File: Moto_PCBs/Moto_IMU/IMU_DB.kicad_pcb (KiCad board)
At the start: 2 copper layers, 60 x 30 mm, 31 parts, among them J1 POWER IN, J2 CANBUS, J3 Conn_01x05_Pin 61300511121, U1 STM32F103C8Tx, U2 IAM-20680HP, U3 SN65HVD230

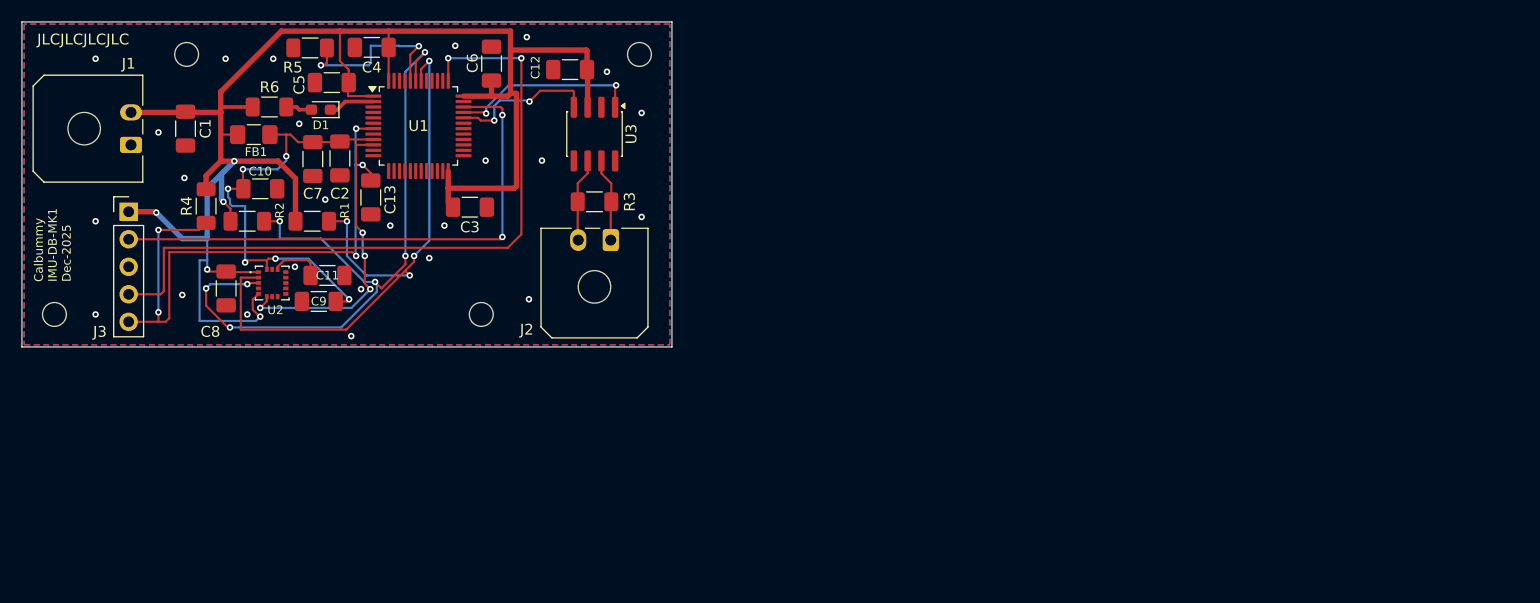
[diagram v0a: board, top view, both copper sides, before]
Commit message: Add files via upload
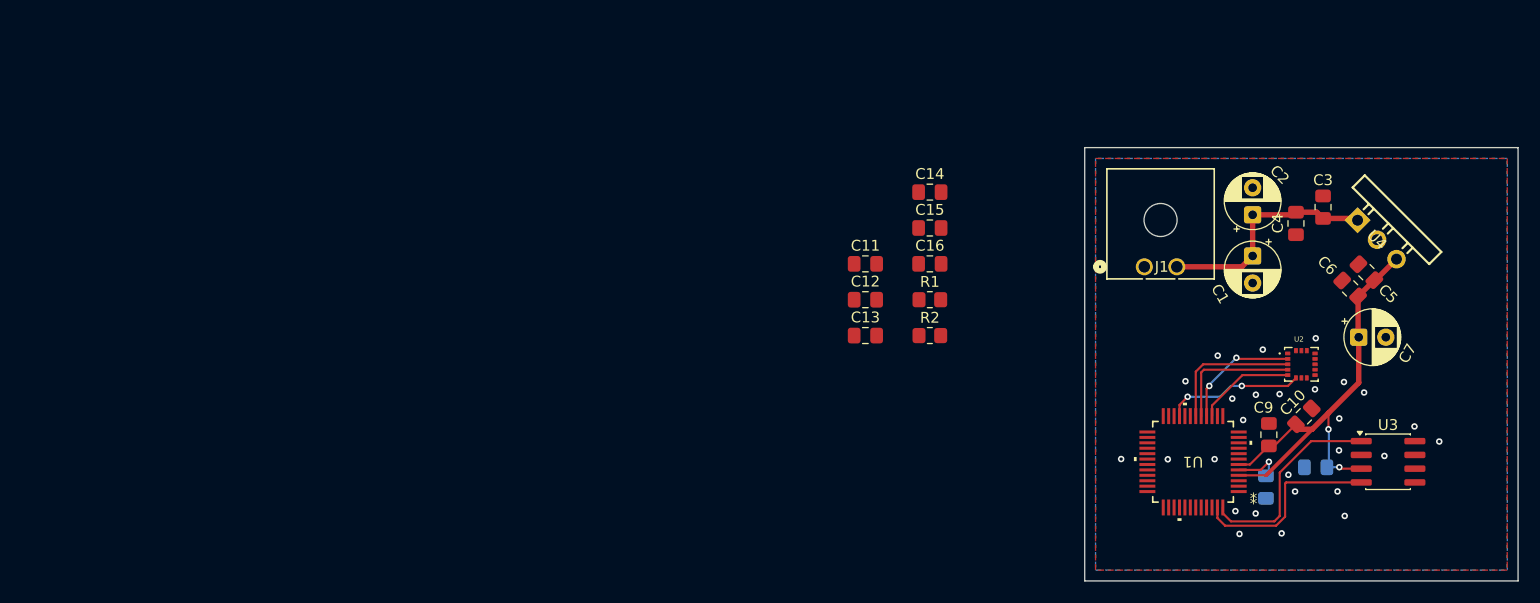
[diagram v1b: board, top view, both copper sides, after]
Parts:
- removed D1: SML-D12P8WT86C, LED_SMD:LED_0603_1608Metric_Pad1.05x0.95mm_HandSolder
- removed FB1: 742792113, Inductor_SMD:L_1206_3216Metric_Pad1.42x1.75mm_HandSolder
- removed J2: CANBUS, Connector_Molex:Molex_Micro-Fit_3.0_43650-0200_1x02_P3.00mm_Horizontal
- removed J3: Conn_01x05_Pin 61300511121, Connector_PinHeader_2.54mm:PinHeader_1x05_P2.54mm_Vertical
- removed R3: RC1206JR-07120RL - OPTIONAL TERM ONLY, Resistor_SMD:R_1206_3216Metric_Pad1.30x1.75mm_HandSolder
- removed R4, R5: RC1206FR-0710KL 10kOhm, Resistor_SMD:R_1206_3216Metric_Pad1.30x1.75mm_HandSolder
- removed R6: RNCP1206FTD1K00 1kOhm, Resistor_SMD:R_1206_3216Metric_Pad1.30x1.75mm_HandSolder
- removed REF** (x4): MountingHole_2.2mm_M2_DIN965, MountingHole:MountingHole_2.2mm_M2_DIN965
- added C14: 10nF, Capacitor_SMD:C_0805_2012Metric_Pad1.18x1.45mm_HandSolder, F.Cu at (108.2, 86.1)
- added C15: .1uF, Capacitor_SMD:C_0805_2012Metric_Pad1.18x1.45mm_HandSolder, F.Cu at (108.2, 89.4)
- added C16: 2.2uF, Capacitor_SMD:C_0805_2012Metric_Pad1.18x1.45mm_HandSolder, F.Cu at (108.2, 92.7)
- added C17: 100nF, Capacitor_SMD:C_0805_2012Metric_Pad1.18x1.45mm_HandSolder, B.Cu at (143.8, 111.5)
- added U4: TPSM84203EAB, TPSM84203EAB:EAB0003A, F.Cu at (149.5, 90.5)
- C1: value CL31B106KQHNFNE 10uF 6.3V -> 100uF; footprint Capacitor_SMD:C_1206_3216Metric_Pad1.33x1.80mm_HandSolder -> Capacitor_THT:CP_Radial_D5.0mm_P2.50mm
- C10: value 885012208013 1uF 10V -> 4.7uF; footprint Capacitor_SMD:C_1206_3216Metric_Pad1.33x1.80mm_HandSolder -> Capacitor_SMD:C_0805_2012Metric_Pad1.18x1.45mm_HandSolder
- C11: value 885012208009 .1uF 10V -> 4.7uF; footprint Capacitor_SMD:C_1206_3216Metric_Pad1.33x1.80mm_HandSolder -> Capacitor_SMD:C_0805_2012Metric_Pad1.18x1.45mm_HandSolder
- C12: value 885012208009 .1uF 10V -> 100nF; footprint Capacitor_SMD:C_1206_3216Metric_Pad1.33x1.80mm_HandSolder -> Capacitor_SMD:C_0805_2012Metric_Pad1.18x1.45mm_HandSolder
- C13: value 885012208009 .1uF 10V -> .47uF; footprint Capacitor_SMD:C_1206_3216Metric_Pad1.33x1.80mm_HandSolder -> Capacitor_SMD:C_0805_2012Metric_Pad1.18x1.45mm_HandSolder
- C2: value C -> 100uF; footprint Capacitor_SMD:C_1206_3216Metric_Pad1.33x1.80mm_HandSolder -> Capacitor_THT:CP_Radial_D5.0mm_P2.50mm
- C3: value 885012208009 .1uF 10V -> .1uF; footprint Capacitor_SMD:C_1206_3216Metric_Pad1.33x1.80mm_HandSolder -> Capacitor_SMD:C_0805_2012Metric_Pad1.18x1.45mm_HandSolder
- C4: value C -> 1uF; footprint Capacitor_SMD:C_1206_3216Metric_Pad1.33x1.80mm_HandSolder -> Capacitor_SMD:C_0805_2012Metric_Pad1.18x1.45mm_HandSolder
- C5: value C -> .1uF; footprint Capacitor_SMD:C_1206_3216Metric_Pad1.33x1.80mm_HandSolder -> Capacitor_SMD:C_0805_2012Metric_Pad1.18x1.45mm_HandSolder
- C6: value C -> 10uF; footprint Capacitor_SMD:C_1206_3216Metric_Pad1.33x1.80mm_HandSolder -> Capacitor_SMD:C_0805_2012Metric_Pad1.18x1.45mm_HandSolder
- C7: value 885012208013 1uF 10V -> 100uF; footprint Capacitor_SMD:C_1206_3216Metric_Pad1.33x1.80mm_HandSolder -> Capacitor_THT:CP_Radial_D5.0mm_P2.50mm
- C8: value 885012208009 .1uF 10V -> 100nF; footprint Capacitor_SMD:C_1206_3216Metric_Pad1.33x1.80mm_HandSolder -> Capacitor_SMD:C_0805_2012Metric_Pad1.18x1.45mm_HandSolder; moved to B.Cu
- C9: value C -> 100nF; footprint Capacitor_SMD:C_1206_3216Metric_Pad1.33x1.80mm_HandSolder -> Capacitor_SMD:C_0805_2012Metric_Pad1.18x1.45mm_HandSolder
- J1: value POWER IN -> Power In 5V; footprint Connector_Molex:Molex_Micro-Fit_3.0_43650-0200_1x02_P3.00mm_Horizontal -> 0436500201:CONN_SD-43650-001_02_MOL
- R1: value RC1206FR-074K7L 4.7kOhm -> 10kOhm; footprint Resistor_SMD:R_1206_3216Metric_Pad1.30x1.75mm_HandSolder -> Resistor_SMD:R_0805_2012Metric_Pad1.20x1.40mm_HandSolder
- R2: value RC1206FR-074K7L 4.7kOhm -> 47kOhm; footprint Resistor_SMD:R_1206_3216Metric_Pad1.30x1.75mm_HandSolder -> Resistor_SMD:R_0805_2012Metric_Pad1.20x1.40mm_HandSolder
- U1: value STM32F103C8Tx -> STM32G0B1CET6N; footprint Package_QFP:LQFP-48_7x7mm_P0.5mm -> STM32G0B1CET6N:LQFP48_STM
- moved C1 99.2 mm to (138.0, 92.0)
- moved C10 98.6 mm to (142.7, 106.8), turned to 45 degrees
- moved C7 97.9 mm to (147.8, 99.5), turned to 0 degrees
- moved C8 97.7 mm to (139.2, 113.3)
- moved C5 97.1 mm to (148.5, 93.5), turned to -45 degrees
- moved U2 95.3 mm to (142.5, 102.0)
- moved J1 94.2 mm to (128.0, 93.0), turned to 180 degrees
- moved C9 88.6 mm to (139.5, 108.5), turned to 90 degrees
- moved C4 86.8 mm to (142.0, 89.0), turned to 90 degrees
- moved C2 84.4 mm to (138.0, 88.2), turned to 90 degrees
- moved C6 81.9 mm to (147.0, 95.0), turned to -45 degrees
- moved U3 79.3 mm to (150.5, 111.0), turned to 0 degrees
- moved C3 78.8 mm to (144.5, 87.5), turned to -90 degrees
- moved U1 77.9 mm to (132.5, 111.0), turned to 180 degrees
- moved R2 63.9 mm to (108.2, 99.3)
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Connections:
- C1 pad 1: Net-(J1-Pin_2) -> /5V IN
- C10 pad 1: Net-(U1-VDDA) -> /3v3 Clean
- C11 pad 1: GND -> /3v3 Clean
- C11 pad 2: Net-(U2-REGOUT) -> GND
- C12 pad 1: Net-(J1-Pin_2) -> /3v3 Clean
- C13 pad 2: Net-(J3-Pin_5) -> Net-(U2-REGOUT)
- C2 pad 1: Net-(U1-VDDA) -> /5V IN
- C3 pad 2: Net-(J1-Pin_2) -> /5V IN
- C4 pad 1: Net-(J1-Pin_2) -> GND
- C4 pad 2: GND -> /5V IN
- C5 pad 2: Net-(J1-Pin_2) -> /3v3 Clean
- C6 pad 1: Net-(J1-Pin_2) -> GND
- C6 pad 2: GND -> /3v3 Clean
- C7 pad 1: Net-(U1-VDDA) -> /3v3 Clean
- C8 pad 2: Net-(J1-Pin_2) -> /3v3 Clean
- C9 pad 1: Net-(U1-VDDA) -> /3v3 Clean
- J1 pad 2: Net-(J1-Pin_2) -> /5V IN
- R1 pad 1: Net-(J1-Pin_2) -> /CS
- R1 pad 2: Net-(U1-PB6) -> GND
- R2 pad 1: Net-(J1-Pin_2) -> /SCK
- R2 pad 2: Net-(U1-PB7) -> GND
- U1 pad 1: Net-(J1-Pin_2) -> unconnected-(U1-PC13-Pad1)
- U1 pad 10: Net-(U1-PA0) -> unconnected-(U1-PF2-NRST-Pad10)
- U1 pad 15: unconnected-(U1-PA5-Pad15) -> /CS
- U1 pad 16: unconnected-(U1-PA6-Pad16) -> /SCK
- U1 pad 17: unconnected-(U1-PA7-Pad17) -> /MISO
- U1 pad 18: unconnected-(U1-PB0-Pad18) -> /MOSI
- U1 pad 2: Net-(D1-K) -> unconnected-(U1-PC14-OSC32_IN-Pad2)
- U1 pad 21: unconnected-(U1-PB10-Pad21) -> /EXTI
- U1 pad 23: GND -> unconnected-(U1-PB11-Pad23)
- U1 pad 24: Net-(J1-Pin_2) -> unconnected-(U1-PB12-Pad24)
- U1 pad 30: unconnected-(U1-PA9-Pad30) -> GND
- U1 pad 31: unconnected-(U1-PA10-Pad31) -> /3v3 Clean
- U1 pad 32: Net-(U1-PA11) -> unconnected-(U1-PA10-Pad32)
- U1 pad 33: Net-(U1-PA12) -> unconnected-(U1-PA11_[PA9]-Pad33)
- U1 pad 34: Net-(J3-Pin_2) -> unconnected-(U1-PA12_[PA10]-Pad34)
- U1 pad 35: GND -> unconnected-(U1-PA13-Pad35)
- U1 pad 36: Net-(J1-Pin_2) -> unconnected-(U1-PA14-BOOT0-Pad36)
- U1 pad 37: Net-(J3-Pin_4) -> unconnected-(U1-PA15-Pad37)
- U1 pad 4: unconnected-(U1-PC15-Pad4) -> /3v3 Clean
- U1 pad 42: Net-(U1-PB6) -> unconnected-(U1-PB3-Pad42)
- U1 pad 43: Net-(U1-PB7) -> unconnected-(U1-PB4-Pad43)
- U1 pad 44: Net-(U1-BOOT0) -> unconnected-(U1-PB5-Pad44)
- U1 pad 47: GND -> Net-(U1-PB8)
- U1 pad 48: Net-(J1-Pin_2) -> Net-(U1-PB9)
- U1 pad 5: unconnected-(U1-PD0-Pad5) -> /3v3 Clean
- U1 pad 6: unconnected-(U1-PD1-Pad6) -> /3v3 Clean
- U1 pad 7: Net-(J3-Pin_5) -> GND
- U1 pad 8: GND -> unconnected-(U1-PF0-OSC_IN-Pad8)
- U1 pad 9: Net-(U1-VDDA) -> unconnected-(U1-PF1-OSC_OUT-Pad9)
- U2 pad 1: Net-(J1-Pin_2) -> /3v3 Clean
- U2 pad 10: unconnected-(U2-RESV9_1215__1-Pad10) -> GND
- U2 pad 11: unconnected-(U2-RESV9_1215__2-Pad11) -> GND
- U2 pad 12: unconnected-(U2-RESV9_1215__3-Pad12) -> GND
- U2 pad 15: unconnected-(U2-RESV9_1215__4-Pad15) -> GND
- U2 pad 16: Net-(U1-VDDA) -> /3v3 Clean
- U2 pad 2: Net-(U1-PB6) -> /SCK
- U2 pad 3: Net-(U1-PB7) -> /MOSI
- U2 pad 4: GND -> /MISO
- U2 pad 5: Net-(J1-Pin_2) -> /CS
- U2 pad 6: Net-(U1-PA0) -> /EXTI
- U2 pad 9: unconnected-(U2-RESV9_1215-Pad9) -> GND
- U3 pad 1: Net-(U1-PA12) -> Net-(U1-PB9)
- U3 pad 3: Net-(J1-Pin_2) -> /3v3 Clean
- U3 pad 4: Net-(U1-PA11) -> Net-(U1-PB8)
- U3 pad 6: Net-(J2-Pin_2) -> unconnected-(U3-CANL-Pad6)
- U3 pad 7: Net-(J2-Pin_1) -> unconnected-(U3-CANH-Pad7)
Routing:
- net Net-(J1-Pin_2): track 163.1 -> 0.00 mm, vias 5 -> 0
- net Net-(U1-PB7): track 66.3 -> 0.00 mm, vias 7 -> 0
- net Net-(J3-Pin_4): track 66.0 -> 0.00 mm, vias 2 -> 0
- net Net-(U1-PB6): track 58.3 -> 0.00 mm, vias 4 -> 0
- net Net-(J3-Pin_5): track 56.3 -> 0.00 mm, vias 5 -> 0
- net Net-(J3-Pin_2): track 50.1 -> 0.00 mm, vias 2 -> 0
- net /3v3 Clean: track 0.00 -> 48.7 mm, vias 0 -> 3
- net Net-(U1-VDDA): track 41.8 -> 0.00 mm, vias 6 -> 0
- net Net-(U1-PA0): track 27.6 -> 0.00 mm, vias 4 -> 0
- net /5V IN: track 0.00 -> 21.6 mm
- net Net-(U1-PB9): track 0.00 -> 19.0 mm
- net Net-(U1-PB8): track 0.00 -> 18.0 mm
- net Net-(U1-PA12): track 17.6 -> 0.00 mm, vias 2 -> 0
- net Net-(U1-BOOT0): track 16.3 -> 0.00 mm, vias 2 -> 0
- net Net-(U1-PA11): track 13.8 -> 0.00 mm, vias 2 -> 0
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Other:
- board size 60 x 30 mm -> 40 x 40 mm
- board text removed: "Calbummy IMU-DB-MK1 Dec-2025"
- board text removed: "JLCJLCJLCJLC"
